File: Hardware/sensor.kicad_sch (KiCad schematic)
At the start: 13 parts

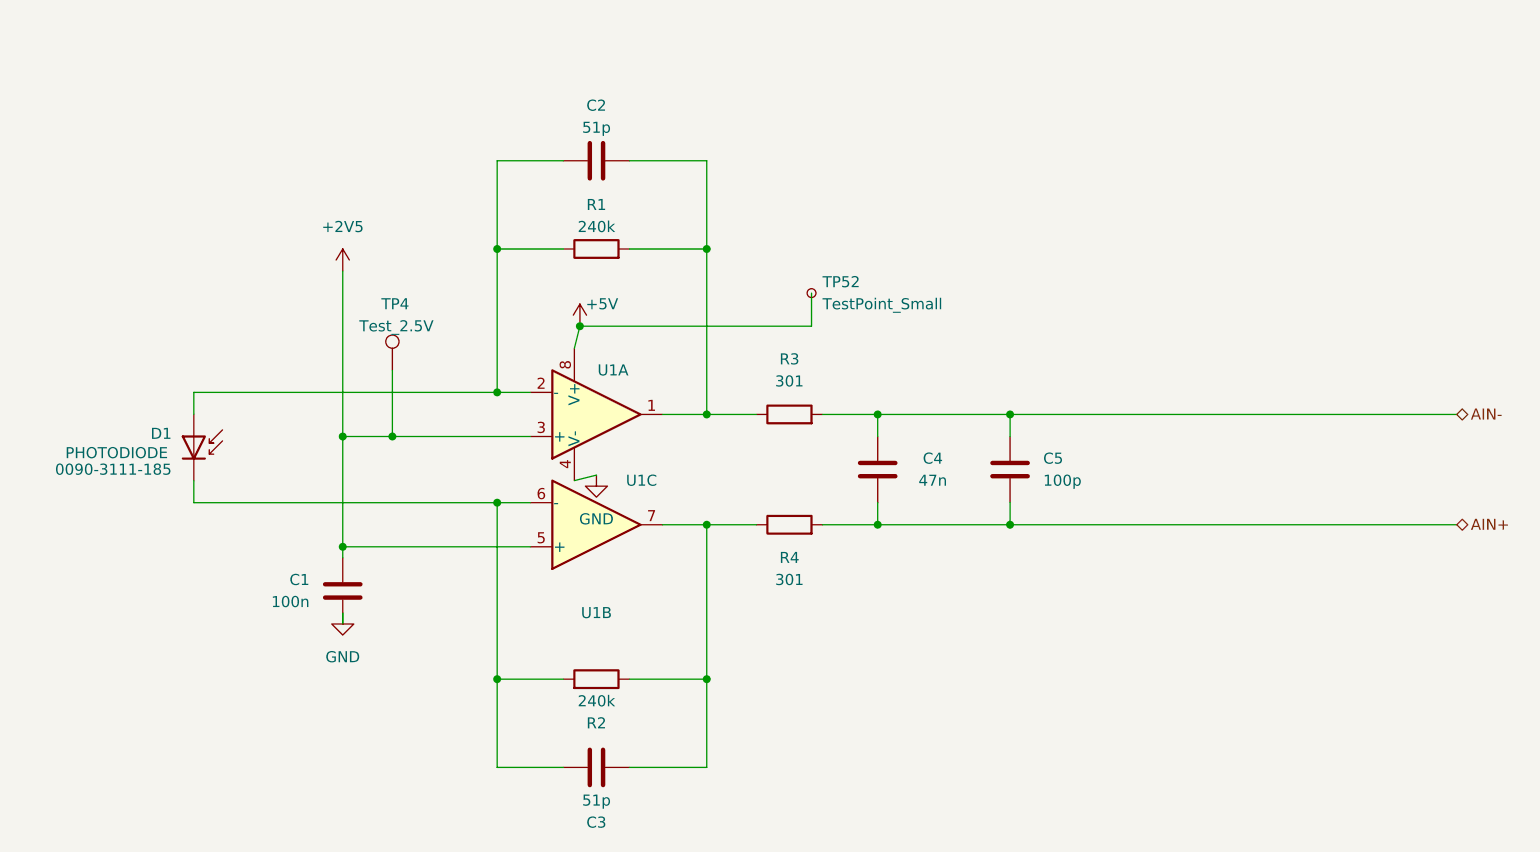
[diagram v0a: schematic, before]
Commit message: Version 0.1
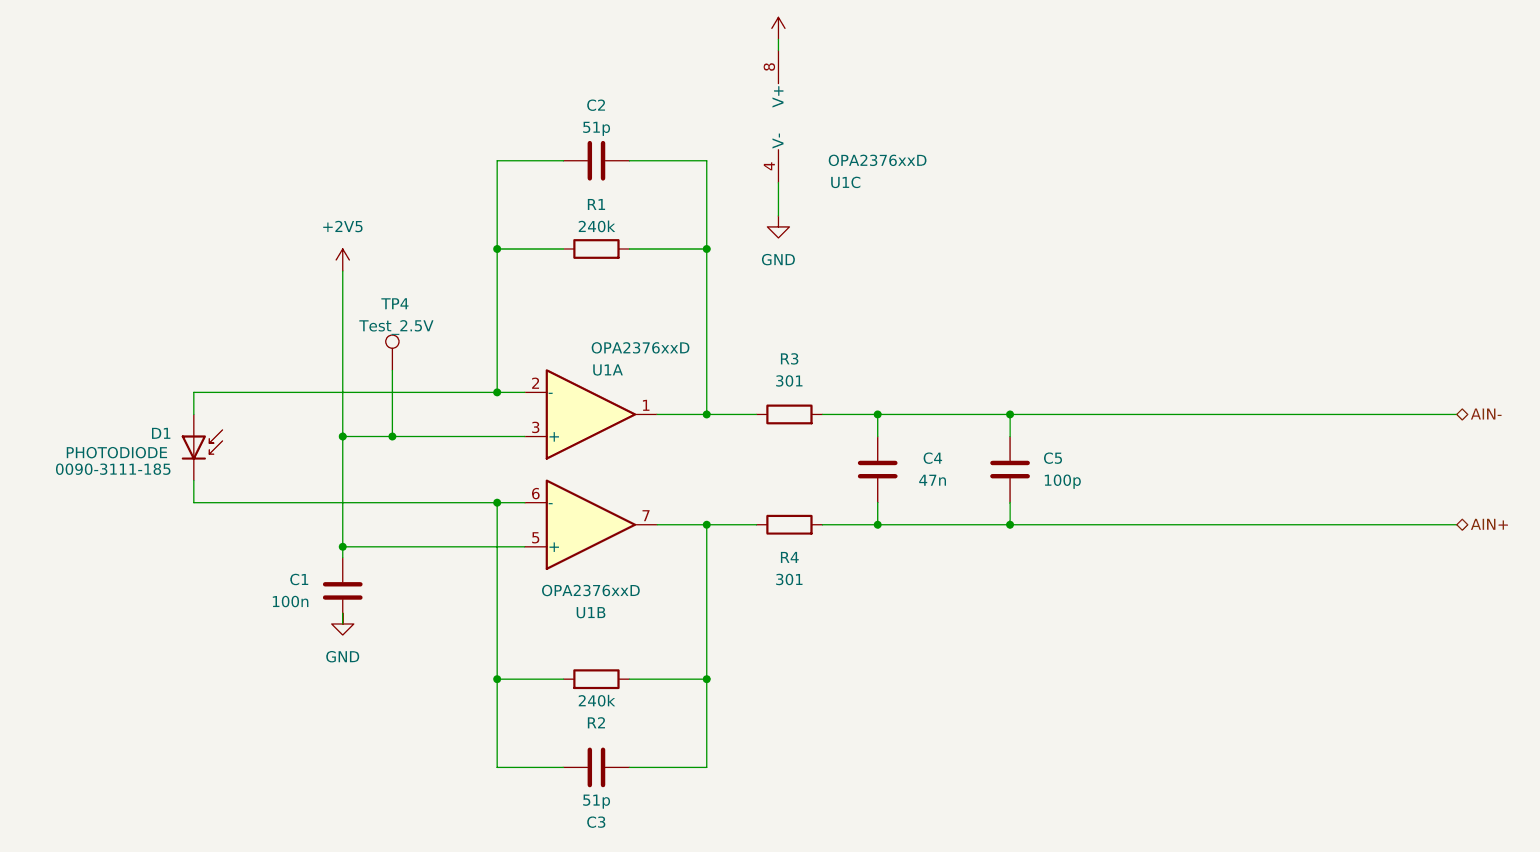
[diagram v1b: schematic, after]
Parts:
- removed TP52: TestPoint_Small, TestPoint:TestPoint_Pad_D1.0mm, symbol Connector:TestPoint_Small
- C1: footprint Capacitor_SMD:C_0805_2012Metric_Pad1.18x1.45mm_HandSolder -> (none)
- C2, C3, C4, C5: footprint Capacitor_SMD:C_0805_2012Metric_Pad1.18x1.45mm_HandSolder -> Capacitor_SMD:C_0603_1608Metric_Pad1.08x0.95mm_HandSolder
- R1, R2, R3, R4: footprint Resistor_SMD:R_0805_2012Metric_Pad1.20x1.40mm_HandSolder -> Resistor_SMD:R_0603_1608Metric_Pad0.98x0.95mm_HandSolder
- U1: value (none) -> OPA2376xxD
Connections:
- net +5V renamed +3V3
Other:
- moved on the sheet: U1A, U1B, U1C
